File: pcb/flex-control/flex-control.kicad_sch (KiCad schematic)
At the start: 3 parts, among them J1 Conn_01x06_MountingPin

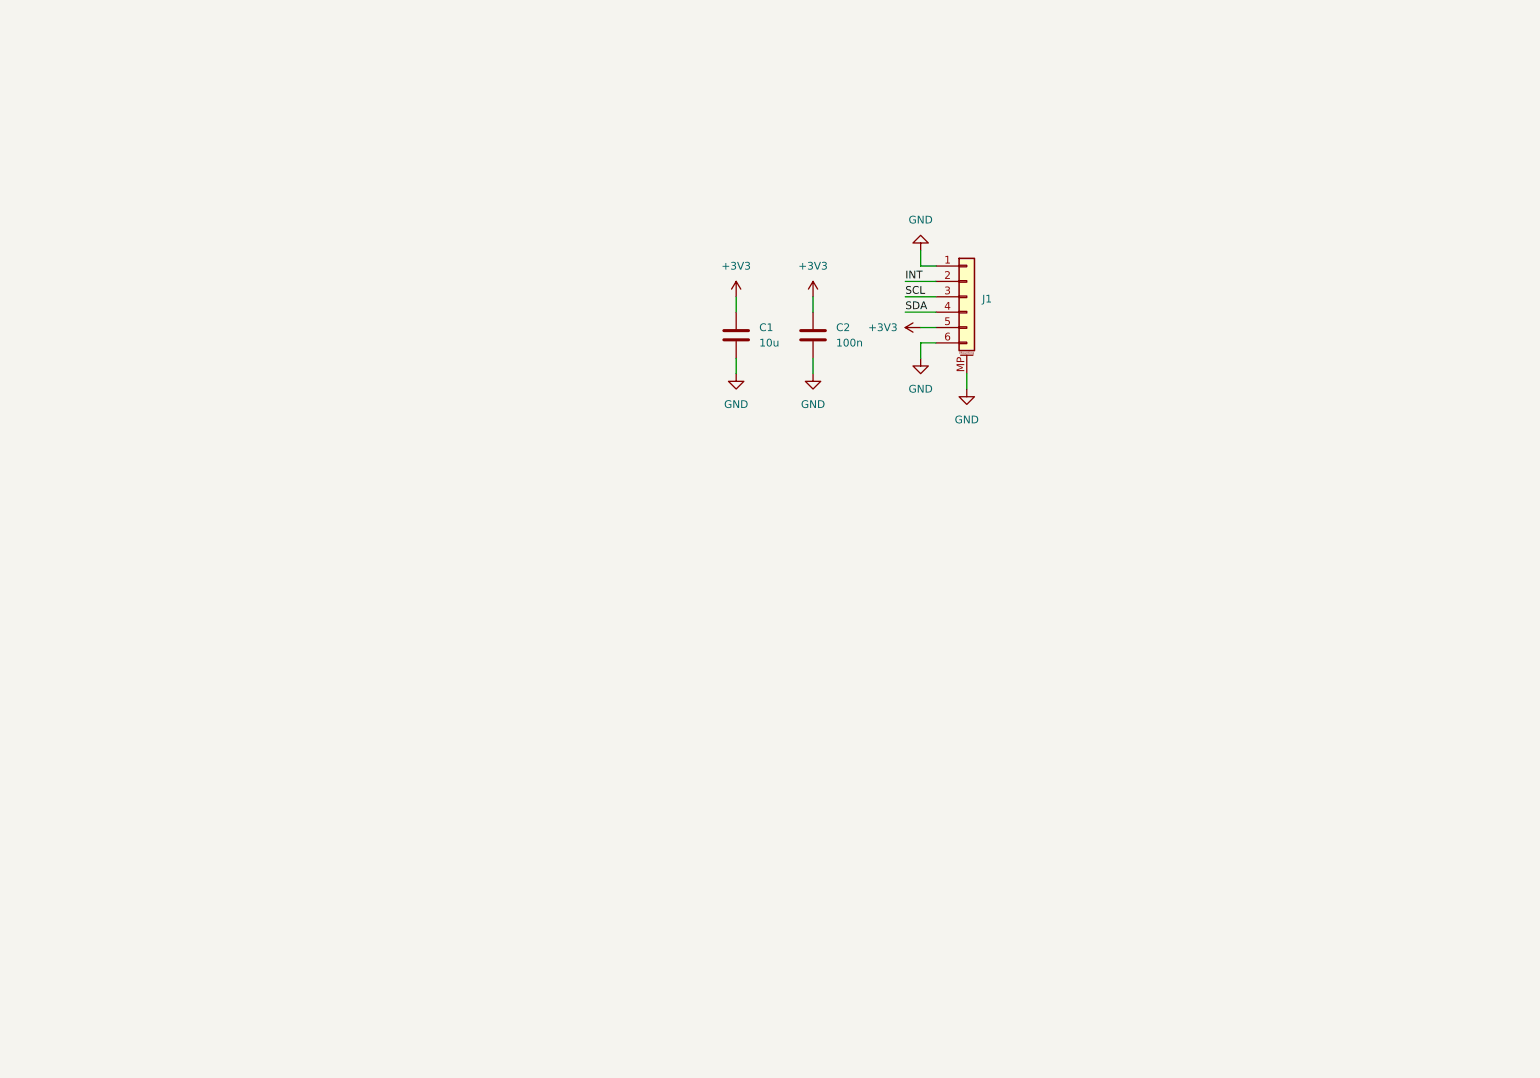
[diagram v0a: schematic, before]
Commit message: Finish routing
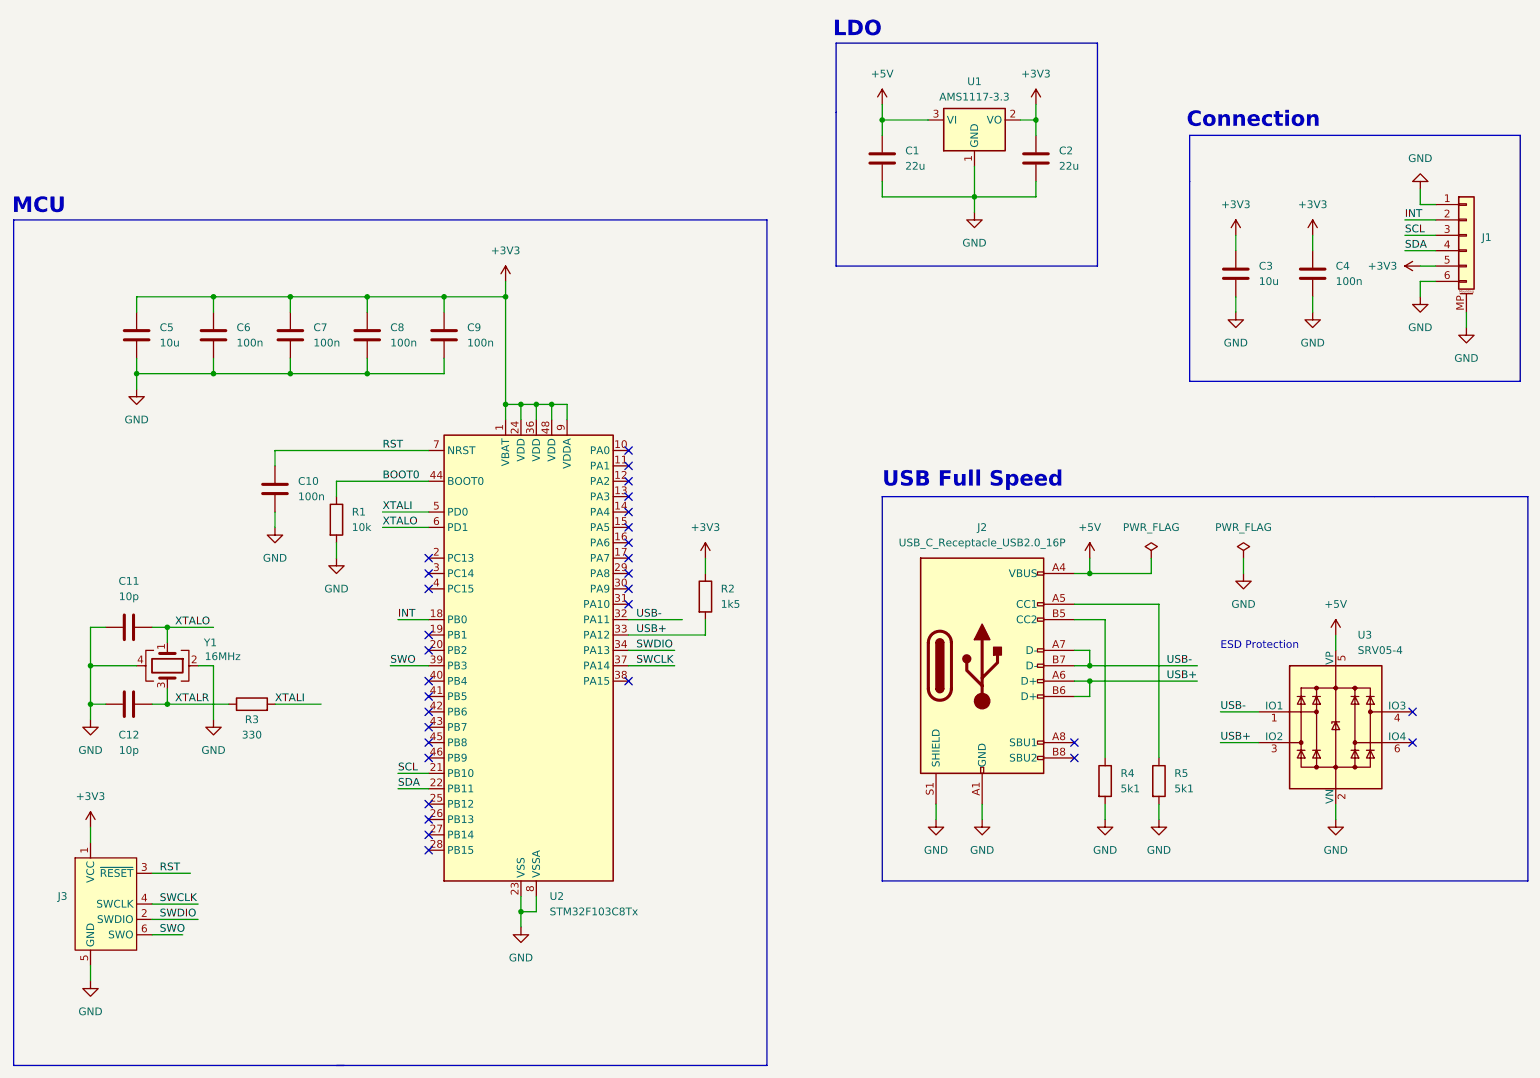
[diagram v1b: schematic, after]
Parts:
- added C10, C4, C6, C7, C8, C9: 100n, Capacitor_SMD:C_0402_1005Metric, symbol Device:C
- added C11, C12: 10p, Capacitor_SMD:C_0402_1005Metric, symbol Device:C
- added C3, C5: 10u, Capacitor_SMD:C_0603_1608Metric, symbol Device:C
- added J2: USB_C_Receptacle_USB2.0_16P, Connector_USB:USB_C_Receptacle_GCT_USB4105-xx-A_16P_TopMnt_Horizontal, symbol Connector:USB_C_Receptacle_USB2.0_16P
- added J3: Conn_ARM_SWD_TagConnect_TC2030-NL, Connector:Tag-Connect_TC2030-IDC-NL_2x03_P1.27mm_Vertical, symbol Connector:Conn_ARM_SWD_TagConnect_TC2030-NL
- added R1: 10k, Resistor_SMD:R_0402_1005Metric, symbol Device:R
- added R2: 1k5, Resistor_SMD:R_0402_1005Metric, symbol Device:R
- added R3: 330, Resistor_SMD:R_0402_1005Metric, symbol Device:R
- added R4, R5: 5k1, Resistor_SMD:R_0402_1005Metric, symbol Device:R
- added U1: AMS1117-3.3, Package_TO_SOT_SMD:SOT-223-3_TabPin2, symbol Regulator_Linear:AMS1117-3.3
- added U2: STM32F103C8Tx, Package_QFP:LQFP-48_7x7mm_P0.5mm, symbol MCU_ST_STM32F1:STM32F103C8Tx
- added U3: SRV05-4, Package_TO_SOT_SMD:SOT-23-6, symbol Power_Protection:SRV05-4
- added Y1: 16MHz, Crystal:Crystal_SMD_3225-4Pin_3.2x2.5mm, symbol Device:Crystal_GND24
- C1: value 10u -> 22u; footprint Capacitor_SMD:C_0603_1608Metric -> Capacitor_SMD:C_0805_2012Metric; LCSC C19702 -> C45783
- C2: value 100n -> 22u; footprint Capacitor_SMD:C_0402_1005Metric -> Capacitor_SMD:C_0603_1608Metric; LCSC C1525 -> C59461
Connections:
- net +3V3: now also C3.1, C4.1, C5.1, C6.1, C7.1, C8.1, C9.1, J3.1 (VCC), R2.1, U1.2 (VO), U2.1 (VBAT), U2.24 (VDD), U2.36 (VDD), U2.48 (VDD), U2.9 (VDDA); no longer C1.1
- net GND: now also C10.2, C11.1, C12.1, C3.2, C4.2, C5.2, C6.2, C7.2, C8.2, C9.2, J2.A1 (GND), J2.A12 (GND), J2.B1 (GND), J2.B12 (GND), J2.S1 (SHIELD), J3.5 (GND), R1.2, R4.2, R5.2, U1.1 (GND), U2.23 (VSS), U2.35 (VSS), U2.47 (VSS), U2.8 (VSSA), U3.2 (VN), Y1.2, Y1.4
- net INT: now also U2.18 (PB0)
- net SCL: now also U2.21 (PB10)
- net SDA: now also U2.22 (PB11)
- new net: J2.B5 (CC2), R4.1
- new net: J2.A5 (CC1), R5.1
- new net +5V: C1.1, J2.A4 (VBUS), J2.A9 (VBUS), J2.B4 (VBUS), J2.B9 (VBUS), U1.3 (VI), U3.5 (VP)
- new net BOOT0: R1.1, U2.44 (BOOT0)
- new net RST: C10.1, J3.3 (~{RESET}), U2.7 (NRST)
- new net SWCLK: J3.4 (SWCLK), U2.37 (PA14)
- new net SWDIO: J3.2 (SWDIO), U2.34 (PA13)
- new net SWO: J3.6 (SWO), U2.39 (PB3)
- new net USB+: J2.A6 (D+), J2.B6 (D+), R2.2, U2.33 (PA12), U3.3 (IO2)
- new net USB-: J2.A7 (D-), J2.B7 (D-), U2.32 (PA11), U3.1 (IO1)
- new net XTALI: R3.2, U2.5 (PD0)
- new net XTALO: C11.2, U2.6 (PD1), Y1.1
- new net XTALR: C12.2, R3.1, Y1.3
- no-connect marks 0 -> 31
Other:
- note added: "Connection"
- note added: "ESD Protection"
- note added: "LDO"
- note added: "MCU"
- note added: "USB Full Speed"
- moved on the sheet: J1

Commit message: Create production files
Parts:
- C3, C5: LCSC C15525 -> C19702
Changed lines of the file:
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@@
 			)
 		)
-		(property "LCSC" "C15525"
+		(property "LCSC" "C19702"
 			(at 222.25 59.69 0)
 			(effects
@@
 			)
 		)
-		(property "LCSC" "C15525"
+		(property "LCSC" "C19702"
 			(at 40.64 69.85 0)
 			(effects
